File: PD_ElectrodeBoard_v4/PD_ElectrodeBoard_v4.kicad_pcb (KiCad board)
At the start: 2 copper layers, 100 x 74 mm, 126 parts, among them J1 Conn_02x32_Odd_Even, J10 Conn_01x02, J11 TopPlate, J2 Conn_02x32_Odd_Even, J3 Conn_01x02, J4 Conn_01x02, J5 Conn_01x02, J6 Conn_01x02, J7 Conn_01x02, J8 Conn_01x02, J9 Conn_01x02, T1 ZNI1000, T2 ZNI1000, T3 ZNI1000, T4 ZNI1000

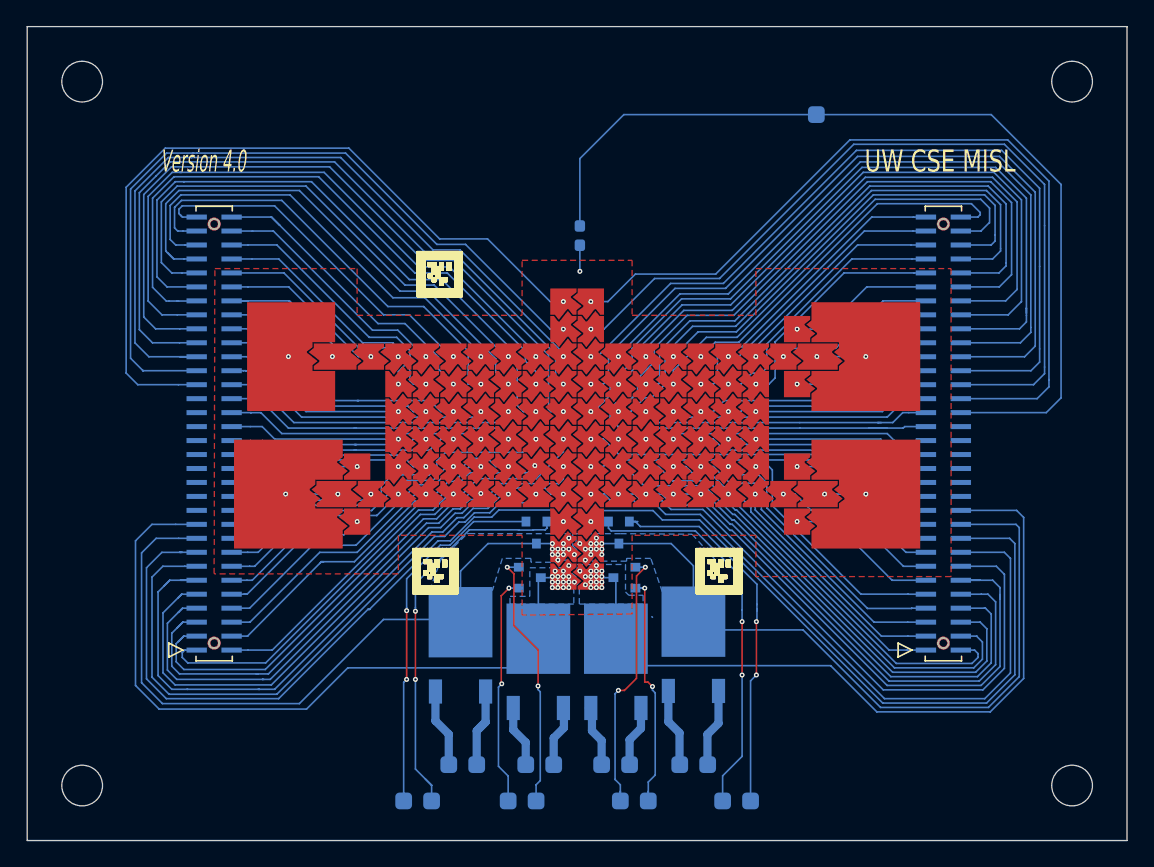
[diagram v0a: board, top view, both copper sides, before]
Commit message: new revision 4.1 of electrode board
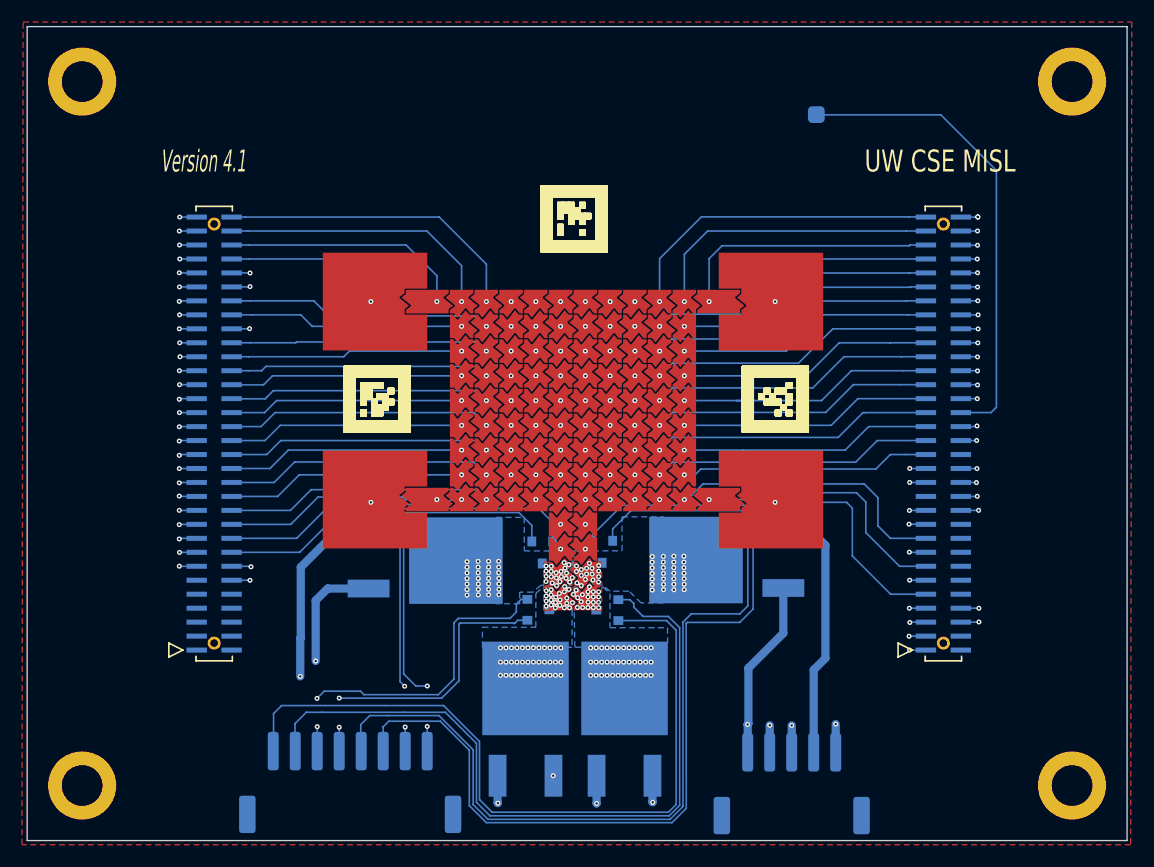
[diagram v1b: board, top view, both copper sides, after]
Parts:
- removed J10, J5, J6, J7, J8, J9: Conn_01x02, PurpleDrop:SMT_PADS_1x2
- removed R5: 0, Resistor_SMD:R_0603_1608Metric_Pad1.05x0.95mm_HandSolder
- added E96: DMFElectrode, electrode_points_1_40deg_tbl, F.Cu at (200.8, 99.8)
- added E97: DMFElectrode, electrode_points_1_40deg_tr, F.Cu at (198.5, 102.0)
- added E98: DMFElectrode, electrode_points_1_40deg_tl, F.Cu at (200.8, 102.0)
- E11: footprint electrode_points_1_40deg_rbl -> electrode_points_1_40deg_trb
- E12, E13, E14: footprint electrode_points_1_40deg_rbl -> electrode_points_1_40deg_trbl
- E15, E29, E43, E57, E85: footprint electrode_points_1_40deg_trb -> electrode_points_1_40deg_trbl
- E20, E30, E40, E50, E60: footprint electrode_points_1_40deg_trbl -> electrode_points_1_40deg_tbl
- E200: footprint electrodes:reservoir_A_2.50mm -> electrodes:reservoir_A_2.25mm
- E201, E202, E203: value ReservoirB -> Reservoir; footprint electrodes:reservoir_B_2.50mm -> electrodes:reservoir_A_2.25mm
- E21, E31, E41, E51, E61: footprint electrode_points_1_40deg_trbl -> electrode_points_1_40deg_trb
- E28, E42, E56, E86: footprint electrode_points_1_40deg_tbl -> electrode_points_1_40deg_trbl
- E7, E8: footprint electrode_points_1_40deg_trbl -> electrode_points_1_40deg_rbl
- E71: footprint electrode_points_1_40deg_trl -> electrode_points_1_40deg_trb
- E72, E73, E74, E75, E76, E79: footprint electrode_points_1_40deg_trl -> electrode_points_1_40deg_trbl
- E80: footprint electrode_points_1_40deg_trl -> electrode_points_1_40deg_tbl
- E87: footprint electrode_points_1_40deg_trb -> electrode_points_1_40deg_trl
- E88: footprint electrode_points_1_40deg_tbl -> electrode_points_1_40deg_trl
- E89: footprint electrode_points_1_40deg_tr -> electrode_points_1_40deg_trl
- E90: footprint electrode_points_1_40deg_tl -> electrode_points_1_40deg_trl
- E91: footprint electrode_points_1_40deg_rb -> electrode_points_1_40deg_trb
- E92: footprint electrode_points_1_40deg_bl -> electrode_points_1_40deg_tbl
- E95: footprint electrode_points_1_40deg_rl -> electrode_points_1_40deg_trb
- G1: renamed from ?; value Fiducial -> AprilTag; footprint PurpleDrop:tag36_11_00000_4.10mm -> PurpleDrop:tag36_11_00004_6.00mm
- G2: renamed from ?; value Fiducial -> AprilTag; footprint PurpleDrop:tag36_11_00000_4.10mm -> PurpleDrop:tag36_11_00005_6.00mm
- G3: renamed from ?; value Fiducial -> AprilTag; footprint PurpleDrop:tag36_11_00000_4.10mm -> PurpleDrop:tag36_11_00006_6.00mm
- H1, H2, H3, H4: footprint PurpleDrop:NPTH3.7 -> PurpleDrop:Keystone-4929
- J3: value Conn_01x02 -> HEAT; footprint PurpleDrop:SMT_PADS_1x2 -> Connector_JST:JST_PH_S5B-PH-SM4-TB_1x05-1MP_P2.00mm_Horizontal
- J4: value Conn_01x02 -> RTD; footprint PurpleDrop:SMT_PADS_1x2 -> Connector_JST:JST_PH_S8B-PH-SM4-TB_1x08-1MP_P2.00mm_Horizontal
- R1, R2, R3, R4: footprint Package_TO_SOT_SMD:TO-252-2 -> PurpleDrop:PWR163_Resistor_DPAK
- moved G2 34.8 mm to (181.8, 83.9)
- moved G1 34.4 mm to (199.7, 67.5)
- moved G3 32.6 mm to (218.0, 83.9)
- moved J4 31.3 mm to (179.4, 118.7)
- moved J3 30.0 mm to (219.5, 118.8)
- moved E95 26.2 mm to (198.5, 99.8)
- moved E42 24.5 mm to (191.8, 84.0)
- moved E29 24.4 mm to (207.5, 79.5)
- moved E41 24.3 mm to (189.5, 84.0)
- moved E30 24.1 mm to (209.8, 79.5)
- moved E92 20.3 mm to (200.8, 95.2)
- moved E91 20.3 mm to (198.5, 95.2)
- moved E14 20.2 mm to (196.2, 77.2)
- moved E84 20.0 mm to (196.2, 93.0)
- moved E94 20.0 mm to (200.8, 97.5)
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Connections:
- E1 pad 1: /P52 -> /P14
- E10 pad 1: /P86 -> /P113
- E11 pad 1: /P82 -> /P8
- E12 pad 1: /P80 -> /P9
- E13 pad 1: /P78 -> /P10
- E14 pad 1: /P77 -> /P19
- E15 pad 1: /P51 -> /P18
- E16 pad 1: /P50 -> /P109
- E17 pad 1: /P48 -> /P108
- E18 pad 1: /P46 -> /P95
- E19 pad 1: /P44 -> /P115
- E2 pad 1: /P49 -> /P15
- E20 pad 1: /P41 -> /P117
- E200 pad 1: /P54 -> /P13
- E200 pad 2: /P55 -> /P12
- E201 pad 1: /P7 -> /P57
- E201 pad 2: /P6 -> /P56
- E202 pad 1: /P73 -> /P114
- E202 pad 2: /P72 -> /P116
- E203 pad 1: /P118 -> /P73
- E203 pad 2: /P119 -> /P75
- E21 pad 1: /P38 -> /P5
- E22 pad 1: /P90 -> /P6
- E23 pad 1: /P87 -> /P23
- E24 pad 1: /P84 -> /P21
- E25 pad 1: /P81 -> /P20
- E26 pad 1: /P79 -> /P107
- E27 pad 1: /P76 -> /P106
- E28 pad 1: /P75 -> /P90
- E29 pad 1: /P58 -> /P118
- E3 pad 1: /P47 -> /P11
- E30 pad 1: /P57 -> /P119
- E31 pad 1: /P56 -> /P3
- E32 pad 1: /P59 -> /P4
- E33 pad 1: /P60 -> /P7
- E34 pad 1: /P42 -> /P24
- E35 pad 1: /P39 -> /P22
- E36 pad 1: /P88 -> /P104
- E37 pad 1: /P83 -> /P105
- E38 pad 1: /P65 -> /P93
- E39 pad 1: /P66 -> /P120
- E4 pad 1: /P45 -> /P16
- E40 pad 1: /P69 -> /P121
- E41 pad 1: /P68 -> /P1
- E42 pad 1: /P67 -> /P2
- E43 pad 1: /P63 -> /P35
- E44 pad 1: /P0 -> /P26
- E45 pad 1: /P1 -> /P25
- E46 pad 1: /P62 -> /P102
- E47 pad 1: /P61 -> /P103
- E48 pad 1: /P8 -> /P66
- E49 pad 1: /P17 -> /P122
- E5 pad 1: /P43 -> /P17
- E51 pad 1: /P85 -> /P63
- E52 pad 1: /P64 -> /P0
- E53 pad 1: /P127 -> /P36
- E54 pad 1: /P124 -> /P28
- E55 pad 1: /P125 -> /P27
- E56 pad 1: /P126 -> /P100
- E57 pad 1: /P3 -> /P101
- E58 pad 1: /P2 -> /P67
- E59 pad 1: /P9 -> /P124
- E6 pad 1: /P40 -> /P111
- E60 pad 1: /P14 -> /P125
- E61 pad 1: /P12 -> /P61
- E62 pad 1: /P15 -> /P62
- E63 pad 1: /P19 -> /P37
- E64 pad 1: /P122 -> /P30
- E65 pad 1: /P109 -> /P29
- E66 pad 1: /P110 -> /P98
- E67 pad 1: /P112 -> /P99
- E68 pad 1: /P114 -> /P69
- E69 pad 1: /P115 -> /P126
- E7 pad 1: /P37 -> /P110
- E70 pad 1: /P116 -> /P127
- E71 pad 1: /P10 -> /P59
- E72 pad 1: /P13 -> /P60
- E73 pad 1: /P16 -> /P38
- E74 pad 1: /P18 -> /P32
- E75 pad 1: /P21 -> /P31
- E76 pad 1: /P22 -> /P91
- E77 pad 1: /P20 -> /P92
- E78 pad 1: /P104 -> /P70
- E79 pad 1: /P105 -> /P64
- E8 pad 1: /P91 -> /P96
- E80 pad 1: /P106 -> /P65
- E81 pad 1: /P107 -> /P55
- E82 pad 1: /P108 -> /P58
- E83 pad 1: /P111 -> /P39
- E84 pad 1: /P113 -> /P34
- E85 pad 1: /P23 -> /P33
- E86 pad 1: /P103 -> /P83
- E87 pad 1: /P24 -> /P74
- E88 pad 1: /P102 -> /P82
- E89 pad 1: /P25 -> /P72
- E9 pad 1: /P89 -> /P112
- E90 pad 1: /P101 -> /P71
- E91 pad 1: /P35 -> /P40
- E92 pad 1: /P93 -> /P76
- E93 pad 1: /P36 -> /P41
- E94 pad 1: /P92 -> /P77
- E95 pad 1: /P53 -> /P54
- J1 pad 1: /P112 -> /P79
- J1 pad 10: /P107 -> /P84
- J1 pad 11: /P117 -> /P74
- J1 pad 12: /P106 -> /P85
- J1 pad 13: /P118 -> /P73
- J1 pad 14: /P105 -> /P86
- J1 pad 15: /P119 -> /P72
- J1 pad 16: /P104 -> /P87
- J1 pad 17: /P120 -> /P71
- J1 pad 18: /P103 -> /P88
- J1 pad 19: /P121 -> /P70
- J1 pad 2: /P111 -> /P80
- J1 pad 20: /P102 -> /P89
- J1 pad 21: /P122 -> /P69
- J1 pad 22: /P101 -> /P90
- J1 pad 23: /P123 -> /P68
- J1 pad 24: /P100 -> /P91
- J1 pad 25: /P124 -> /P67
- J1 pad 26: /P99 -> /P92
- J1 pad 27: /P125 -> /P66
- J1 pad 28: /P98 -> /P93
- J1 pad 29: /P126 -> /P65
- J1 pad 3: /P113 -> /P78
- J1 pad 30: /P97 -> /P94
- J1 pad 31: /P127 -> /P64
- J1 pad 32: /P96 -> /P95
- J1 pad 33: /P64 -> /P127
- J1 pad 34: /P95 -> /P96
- J1 pad 35: /P65 -> /P126
- J1 pad 36: /P94 -> /P97
- J1 pad 37: /P66 -> /P125
- J1 pad 38: /P93 -> /P98
- J1 pad 39: /P67 -> /P124
- J1 pad 4: /P110 -> /P81
- J1 pad 40: /P92 -> /P99
- J1 pad 41: /P68 -> /P123
- J1 pad 42: /P91 -> /P100
- J1 pad 43: /P69 -> /P122
- J1 pad 44: /P90 -> /P101
- J1 pad 45: /P70 -> /P121
- J1 pad 46: /P89 -> /P102
- J1 pad 47: /P71 -> /P120
- J1 pad 48: /P88 -> /P103
- J1 pad 49: /P72 -> /P119
- J1 pad 5: /P114 -> /P77
- J1 pad 50: /P87 -> /P104
- J1 pad 51: /P73 -> /P118
- J1 pad 52: /P86 -> /P105
- J1 pad 53: /P74 -> /P117
- J1 pad 54: /P85 -> /P106
- J1 pad 55: /P75 -> /P116
- J1 pad 56: /P84 -> /P107
- J1 pad 57: /P76 -> /P115
- J1 pad 58: /P83 -> /P108
- J1 pad 59: /P77 -> /P114
- J1 pad 6: /P109 -> /P82
- J1 pad 60: /P82 -> /P109
- J1 pad 61: /P78 -> /P113
- J1 pad 62: /P81 -> /P110
- J1 pad 63: /P79 -> /P112
- J1 pad 64: /P80 -> /P111
- J1 pad 7: /P115 -> /P76
- J1 pad 8: /P108 -> /P83
- J1 pad 9: /P116 -> /P75
- J11 pad 1: /P94 -> /P97
- J2 pad 1: /P16 -> /P47
- J2 pad 10: /P11 -> /P52
- J2 pad 11: /P21 -> /P42
- J2 pad 12: /P10 -> /P53
- J2 pad 13: /P22 -> /P41
- J2 pad 14: /P9 -> /P54
- J2 pad 15: /P23 -> /P40
- J2 pad 16: /P8 -> /P55
- J2 pad 17: /P24 -> /P39
- J2 pad 18: /P7 -> /P56
- J2 pad 19: /P25 -> /P38
- J2 pad 2: /P15 -> /P48
- J2 pad 20: /P6 -> /P57
- J2 pad 21: /P26 -> /P37
- J2 pad 22: /P5 -> /P58
- J2 pad 23: /P27 -> /P36
- J2 pad 24: /P4 -> /P59
- J2 pad 25: /P28 -> /P35
- J2 pad 26: /P3 -> /P60
- J2 pad 27: /P29 -> /P34
- J2 pad 28: /P2 -> /P61
- J2 pad 29: /P30 -> /P33
- J2 pad 3: /P17 -> /P46
- J2 pad 30: /P1 -> /P62
- J2 pad 31: /P31 -> /P32
- J2 pad 32: /P0 -> /P63
- J2 pad 33: /P32 -> /P31
- J2 pad 34: /P63 -> /P0
- J2 pad 35: /P33 -> /P30
- J2 pad 36: /P62 -> /P1
- J2 pad 37: /P34 -> /P29
- J2 pad 38: /P61 -> /P2
- J2 pad 39: /P35 -> /P28
- J2 pad 4: /P14 -> /P49
- J2 pad 40: /P60 -> /P3
- J2 pad 41: /P36 -> /P27
- J2 pad 42: /P59 -> /P4
- J2 pad 43: /P37 -> /P26
- J2 pad 44: /P58 -> /P5
- J2 pad 45: /P38 -> /P25
- J2 pad 46: /P57 -> /P6
- J2 pad 47: /P39 -> /P24
- J2 pad 48: /P56 -> /P7
- J2 pad 49: /P40 -> /P23
- J2 pad 5: /P18 -> /P45
- J2 pad 50: /P55 -> /P8
- J2 pad 51: /P41 -> /P22
- J2 pad 52: /P54 -> /P9
- J2 pad 53: /P42 -> /P21
- J2 pad 54: /P53 -> /P10
- J2 pad 55: /P43 -> /P20
- J2 pad 56: /P52 -> /P11
- J2 pad 57: /P44 -> /P19
- J2 pad 58: /P51 -> /P12
- J2 pad 59: /P45 -> /P18
- J2 pad 6: /P13 -> /P50
- J2 pad 60: /P50 -> /P13
- J2 pad 61: /P46 -> /P17
- J2 pad 62: /P49 -> /P14
- J2 pad 63: /P47 -> /P16
- J2 pad 64: /P48 -> /P15
- J2 pad 7: /P19 -> /P44
- J2 pad 8: /P12 -> /P51
- J2 pad 9: /P20 -> /P43
- J4 pad 1: Net-(J4-Pad1) -> /RTD1_A
- J4 pad 2: Net-(J4-Pad2) -> /RTD1_B
- R1 pad 2: /P24 -> /P54
- R1 pad 3: Net-(J3-Pad2) -> Net-(J3-Pad5)
- R2 pad 1: Net-(J4-Pad1) -> Net-(J3-Pad2)
- R2 pad 2: /P102 -> /P78
- R2 pad 3: Net-(J4-Pad2) -> Net-(J3-Pad5)
- R3 pad 1: Net-(J5-Pad1) -> Net-(J3-Pad3)
- R3 pad 2: /P25 -> /P53
- R3 pad 3: Net-(J5-Pad2) -> Net-(J3-Pad5)
- R4 pad 1: Net-(J6-Pad1) -> Net-(J3-Pad4)
- R4 pad 2: /P101 -> /P79
- R4 pad 3: Net-(J6-Pad2) -> Net-(J3-Pad5)
- T1 pad 1: Net-(J7-Pad1) -> /RTD1_A
- T1 pad 2: Net-(J7-Pad2) -> /RTD1_B
- T1 pad 3: /P24 -> /P54
- T2 pad 1: Net-(J8-Pad1) -> /RTD2_A
- T2 pad 2: Net-(J8-Pad2) -> /RTD2_B
- T2 pad 3: /P102 -> /P78
- T3 pad 1: Net-(J9-Pad1) -> /RTD3_A
- T3 pad 2: Net-(J9-Pad2) -> /RTD3_B
- T3 pad 3: /P25 -> /P53
- T4 pad 1: Net-(J10-Pad1) -> /RTD4_A
- T4 pad 2: Net-(J10-Pad2) -> /RTD4_B
- T4 pad 3: /P101 -> /P79
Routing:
- net Net-(J3-Pad5): track 0.00 -> 92.1 mm, vias 0 -> 4
- net /RTD2_A: track 0.00 -> 86.6 mm
- net /RTD2_B: track 0.00 -> 85.2 mm
- net /P94: track 83.2 -> 0.00 mm
- net /RTD4_B: track 0.00 -> 69.3 mm
- net /P88: track 69.2 -> 0.00 mm, vias 1 -> 0
- net /RTD4_A: track 0.00 -> 68.4 mm
- net /P89: track 65.4 -> 0.00 mm, vias 1 -> 0
- net /P85: track 62.0 -> 0.00 mm, vias 1 -> 0
- net /P87: track 61.8 -> 0.00 mm, vias 1 -> 0
- net /P42: track 57.5 -> 0.00 mm, vias 1 -> 0
- net Net-(J3-Pad1): track 7.81 -> 63.5 mm, vias 0 -> 2
- net /P86: track 55.4 -> 0.00 mm, vias 1 -> 0
- net /P84: track 52.6 -> 0.00 mm, vias 1 -> 0
- net /P44: track 47.8 -> 0.00 mm, vias 1 -> 0
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- added copper zone on B.Cu, net /P53
- added copper zone on F.Cu, net /P53
- added copper zone on In1.Cu, net /P53
- added copper zone on In2.Cu, net /P53
- added copper zone on B.Cu, net /P54
- added copper zone on F.Cu, net /P54
- added copper zone on In1.Cu, net /P54
- added copper zone on In2.Cu, net /P54
- added copper zone on B.Cu, net /P78
- added copper zone on F.Cu, net /P78
- added copper zone on In1.Cu, net /P78
- added copper zone on In2.Cu, net /P78
- added copper zone on B.Cu, net /P79
- added copper zone on F.Cu, net /P79
- added copper zone on In1.Cu, net /P79
- added copper zone on In2.Cu, net /P79
- added copper zone on F.Cu, net /POUR
- removed copper zone on F.Cu, net /GUARD
- removed copper zone on B.Cu, net /P101
- removed copper zone on B.Cu, net /P102
- removed copper zone on B.Cu, net /P24
- removed copper zone on B.Cu, net /P25
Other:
- copper layers 2 -> 4
- board text added: "NOTES: (UNLESS OTHERWISE SPECIFIED) 1. STANDARD A. PCB TO BE FABRICATED IN ACCORDANCE WITH IPC-6012, CLASS 2 2. MATERIAL A. FR-4 B. FINISHED THICKNESS TO BE 0.062" 3. SURFACE FINISH A. ENIG 4. HOLES A. ALL PLATED HOLES TO BE FILLED WITH CONDUCTIVE EPOXY FILL AND PLATED OVER FOR VIA-IN-PAD ON TOP LAYER 5. SOLDERMASK A. SOLDERMASK OVER BARE COPPER ON TOP AND BOTTOM SIDES ACCODING TO SUPPLIED ARTWOR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"
- board text added: "Version 4.1"
- board text removed: "NOTES: (UNLESS OTHERWISE SPECIFIED) 1. STANDARD A. PCB TO BE FABRICATED IN ACCORDANCE WITH IPC-6012, CLASS 2 2. MATERIAL A. FR-4 B. FINISHED THICKNESS TO BE 0.31" 3. SURFACE FINISH A. ENIG 4. HOLES A. ALL PLATED HOLES TO BE FILLED WITH CONDUCTIVE EPOXY FILL AND PLATED OVER FOR VIA-IN-PAD ON TOP LAYER 5. SOLDERMASK A. SOLDERMASK OVER BARE COPPER ON TOP AND BOTTOM SIDES ACCODING TO SUPPLIED ARTWORK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"
- board text removed: "Version 4.0"
